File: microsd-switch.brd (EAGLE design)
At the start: 34.8 x 48.2 mm, 12 parts, among them IC1 SN74CBT3257D, IC2 SN74CBT3257D, U1 USD-SOCKETNEW

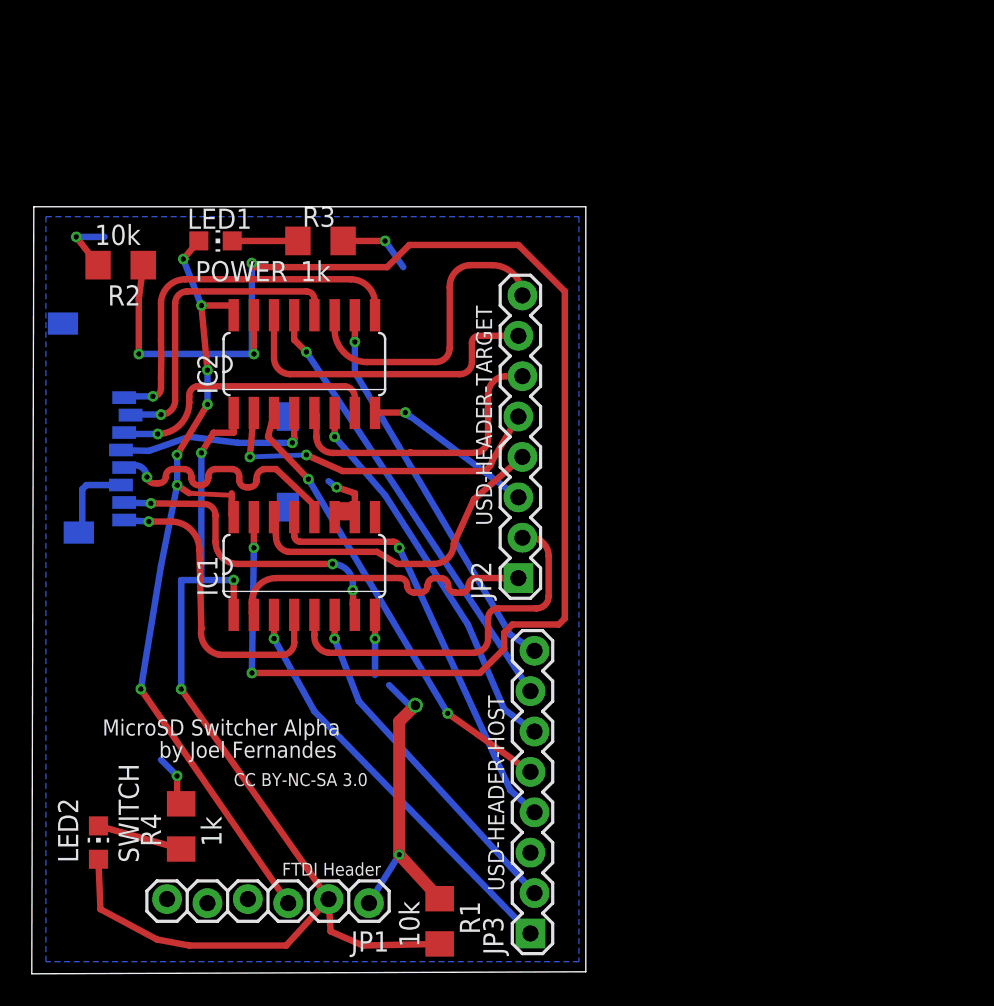
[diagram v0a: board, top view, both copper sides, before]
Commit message: Revert "MicroSD Switch Rev Alpha released"
This reverts commit e0d3fcd5b1a8d34c9a3cecba9fd5e98c93932393.
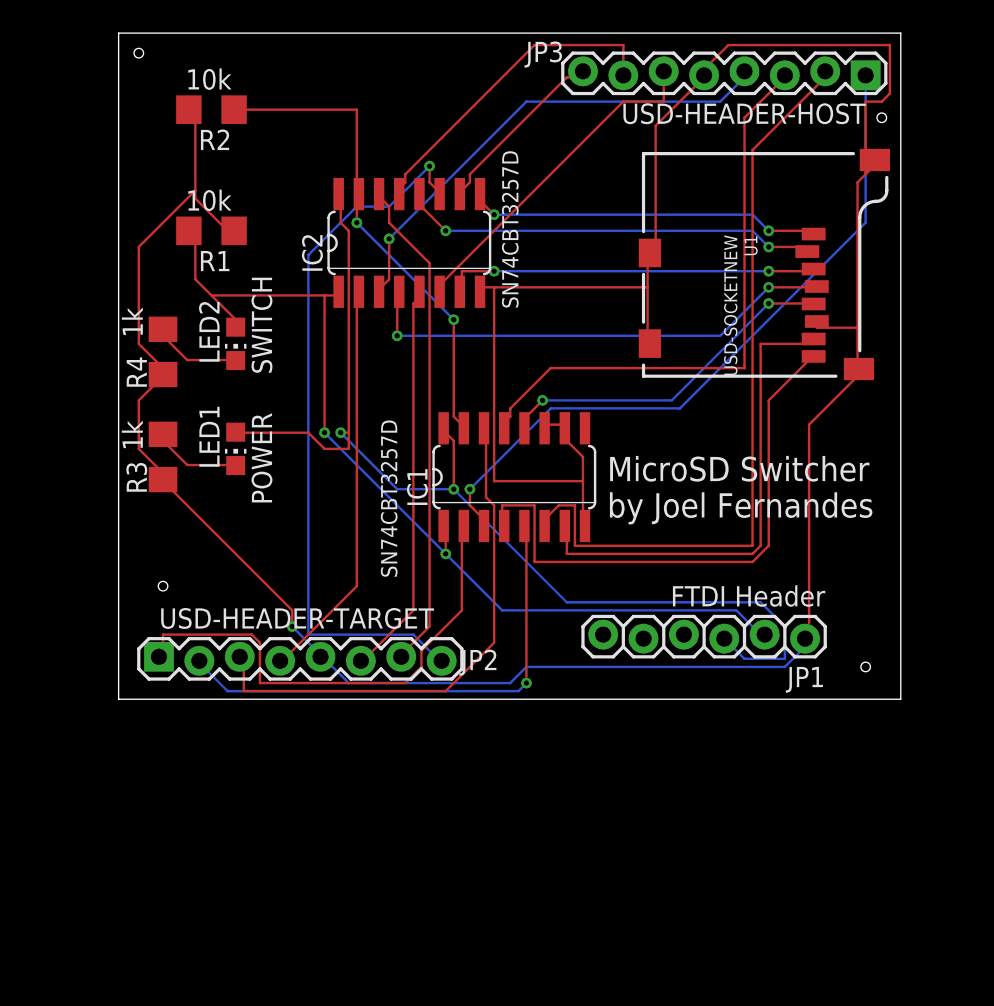
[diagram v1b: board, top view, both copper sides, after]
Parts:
- moved JP3 58.0 mm to (81.3, 77.5), turned to 180 degrees
- moved R1 45.7 mm to (40.1, 67.6), turned to 180 degrees
- moved LED2 32.5 mm to (41.7, 60.5), turned to 180 degrees
- moved JP1 32.1 mm to (77.5, 41.9)
- moved R4 29.9 mm to (37.1, 59.9), turned to 270 degrees
- moved U1 24.3 mm to (67.3, 58.4), flipped to the top
- moved JP2 23.3 mm to (36.8, 40.6), turned to 0 degrees
- moved R3 16.8 mm to (37.1, 53.3), turned to 270 degrees
- moved IC1 14.3 mm to (59.2, 52.1)
- moved LED1 13.1 mm to (41.7, 53.8), turned to 180 degrees
- moved R2 11.3 mm to (40.1, 75.2)
- moved IC2 10.1 mm to (52.6, 66.8)
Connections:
- net CLK-Y renamed N$1
- net CLK-A: now also JP2.3; no longer JP2.4
- net CLK-B: now also JP3.3; no longer JP3.4
- net GND: now also JP2.5, JP3.5; no longer JP2.3, JP3.3
- net VDD-A: now also JP2.4; no longer JP2.5
- net VDD-B: now also JP3.4; no longer JP3.5
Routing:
- net GND: track 61.4 -> 191.6 mm, vias 8 -> 1
- net OE: track 94.8 -> 30.6 mm, vias 5 -> 2
- net DAT0-B: track 22.1 -> 48.2 mm, vias 1 -> 0
- net DAT2-A: track 19.1 -> 44.8 mm, vias 0 -> 1
- net DAT1-B: track 26.2 -> 43.9 mm
- net N$2: track 12.9 -> 30.5 mm, vias 1 -> 2
- net DAT1-Y: track 19.2 -> 35.2 mm, vias 1 -> 0
- net VCC: track 53.6 -> 67.8 mm, vias 7 -> 2
- net DAT2-B: track 24.6 -> 11.5 mm, vias 1 -> 0
- net CLK-A: track 20.7 -> 33.1 mm
- net DAT1-A: track 19.8 -> 30.9 mm
- net DAT0-Y: track 19.4 -> 30.4 mm, vias 3 -> 0
- net DAT3-A: track 20.2 -> 31.1 mm
- net CLK-B: track 26.9 -> 36.7 mm, vias 1 -> 0
- net HOSTSELECT: track 68.9 -> 59.3 mm, vias 3 -> 2
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- removed copper zone on layer 16, net GND
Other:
- board size 34.8 x 48.2 mm -> 49.2 x 41.9 mm
- board text added: "MicroSD Switcher by Joel Fernandes"
- board text removed: "CC BY-NC-SA 3.0"
- board text removed: "MicroSD Switcher Alpha"
- board text removed: "by Joel Fernandes"
